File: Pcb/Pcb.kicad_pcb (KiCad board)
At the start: 2 copper layers, 152.3 x 104.7 mm, 135 parts, among them J1 TRRS, Q1 2N7002, SW1 SW_Push, SW10 SW_Push, SW11 SW_Push, SW12 SW_Push, SW13 SW_Push, SW14 SW_Push, SW15 SW_Push, SW16 SW_Push, SW17 SW_Push, SW18 SW_Push, SW19 SW_Push, SW2 SW2, SW20 SW_Push, SW21 SW_Push, SW22 SW_Push, SW23 SW_Push, SW24 SW_Push, SW25 SW_Push, SW26 SW_Push, SW27 SW_Push, SW28 SW_Push, SW29 SW_Push, SW3 SW_Push, SW4 SW_Push, SW5 SW_Push, SW6 SW_Push, SW7 SW_Push, SW8 SW_Push, SW9 SW_Push, U1 ProMicro

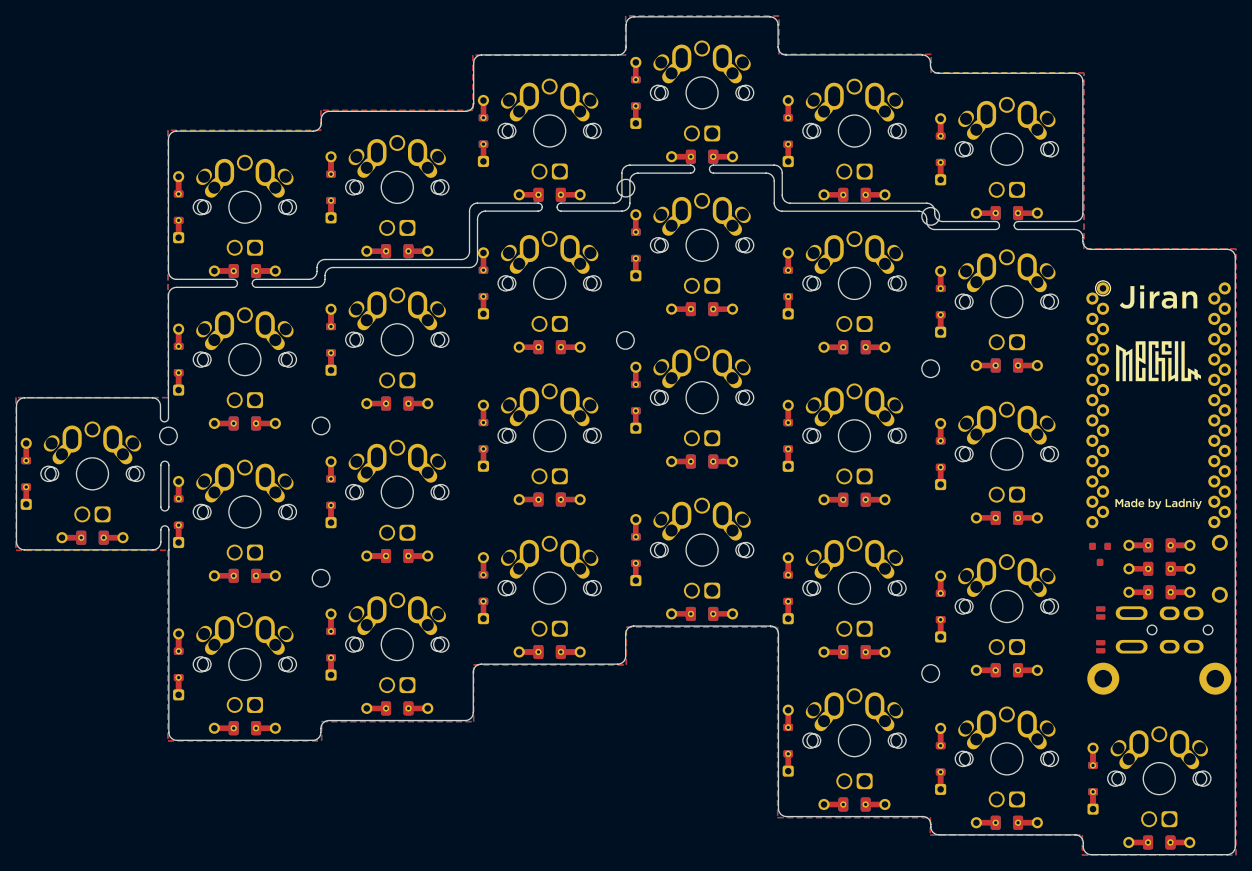
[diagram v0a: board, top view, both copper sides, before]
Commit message: Route tracks
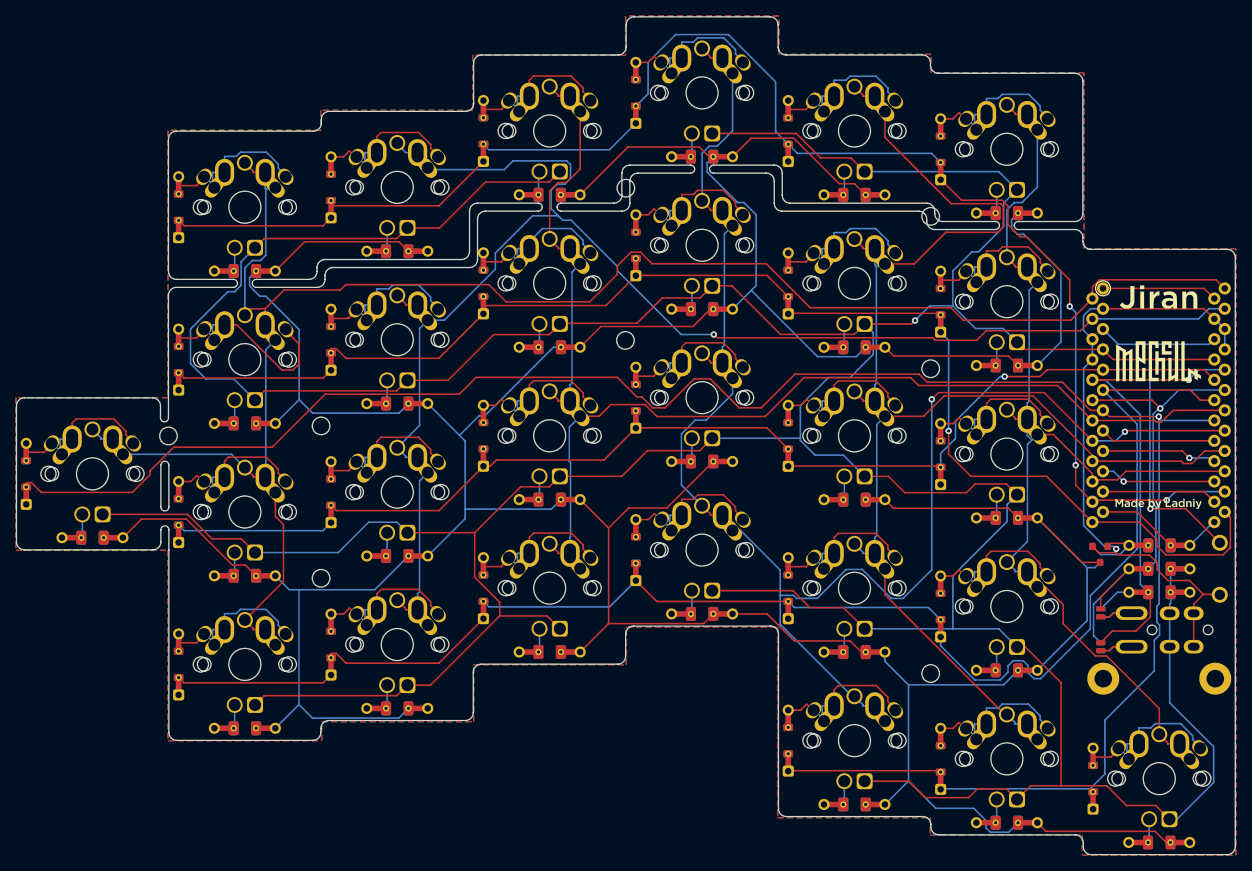
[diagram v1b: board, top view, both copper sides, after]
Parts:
- renumbered LG*** to LG1, LG*** to LG2
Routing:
- net VCC: track 0.00 -> 629.7 mm, vias 0 -> 1
- net /LEDOut: track 0.00 -> 587.6 mm
- net /rowE: track 0.00 -> 262.4 mm, vias 0 -> 1
- net /col0: track 0.00 -> 231.9 mm
- net /col1: track 0.00 -> 199.0 mm, vias 0 -> 1
- net /rowA: track 0.00 -> 197.9 mm, vias 0 -> 3
- net /col3: track 0.00 -> 196.4 mm, vias 0 -> 2
- net /rowD: track 0.00 -> 191.5 mm
- net /col4: track 0.00 -> 176.9 mm
- net /rowB: track 0.00 -> 176.6 mm, vias 0 -> 1
- net /col2: track 0.00 -> 162.4 mm
- net /rowC: track 0.00 -> 156.7 mm, vias 0 -> 1
- net /col5: track 0.00 -> 134.3 mm
- net GND: track 0.00 -> 80.5 mm, vias 0 -> 1
- net SDA: track 0.00 -> 65.0 mm, vias 0 -> 1
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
